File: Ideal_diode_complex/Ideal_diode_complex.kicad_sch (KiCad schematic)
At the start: 34 parts, among them CN1 24_243_1, CN2 24_243_1, CN3 24_243_2, CN4 24_243_2, Q1 SI7336ADP-T1-GE3-HXY, U1 TPS61041DBVR, U2 LTC4352CMS_TRPBF

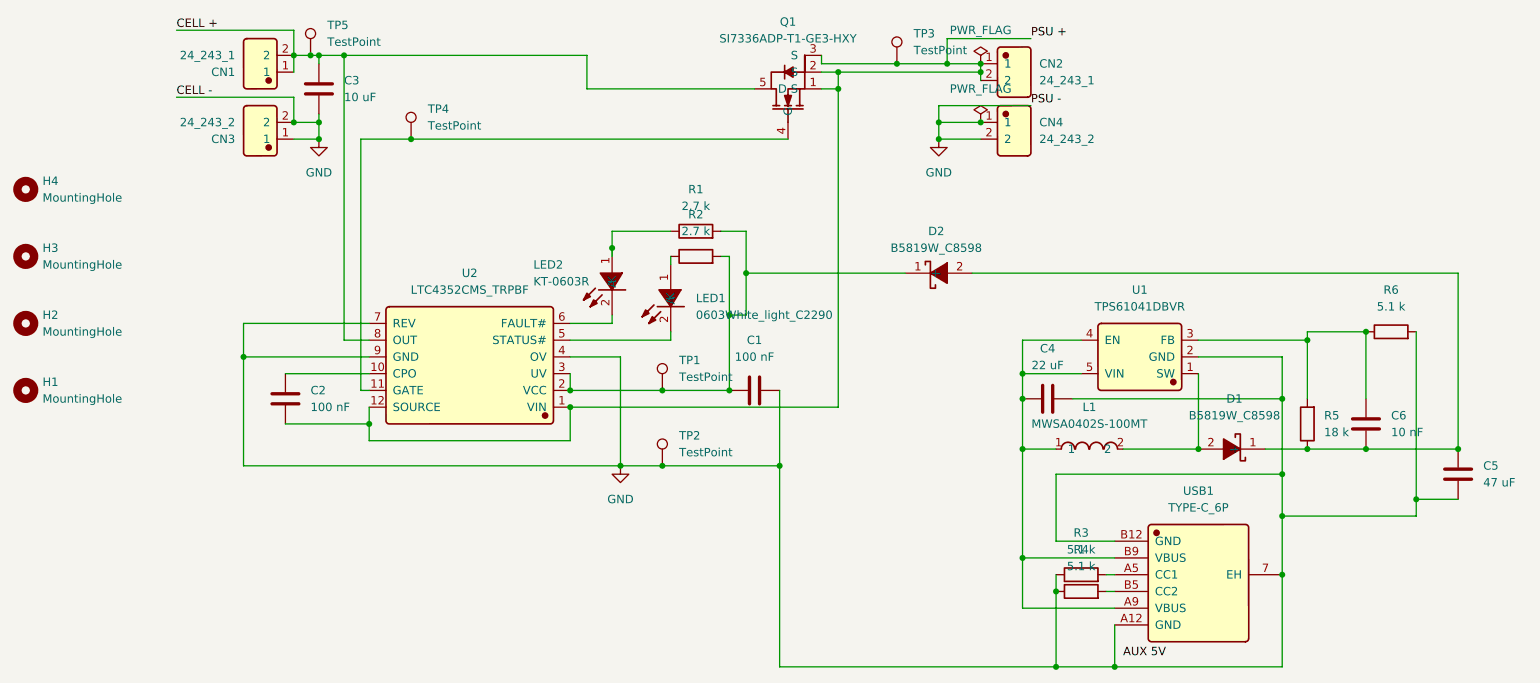
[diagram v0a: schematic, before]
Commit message: Final design
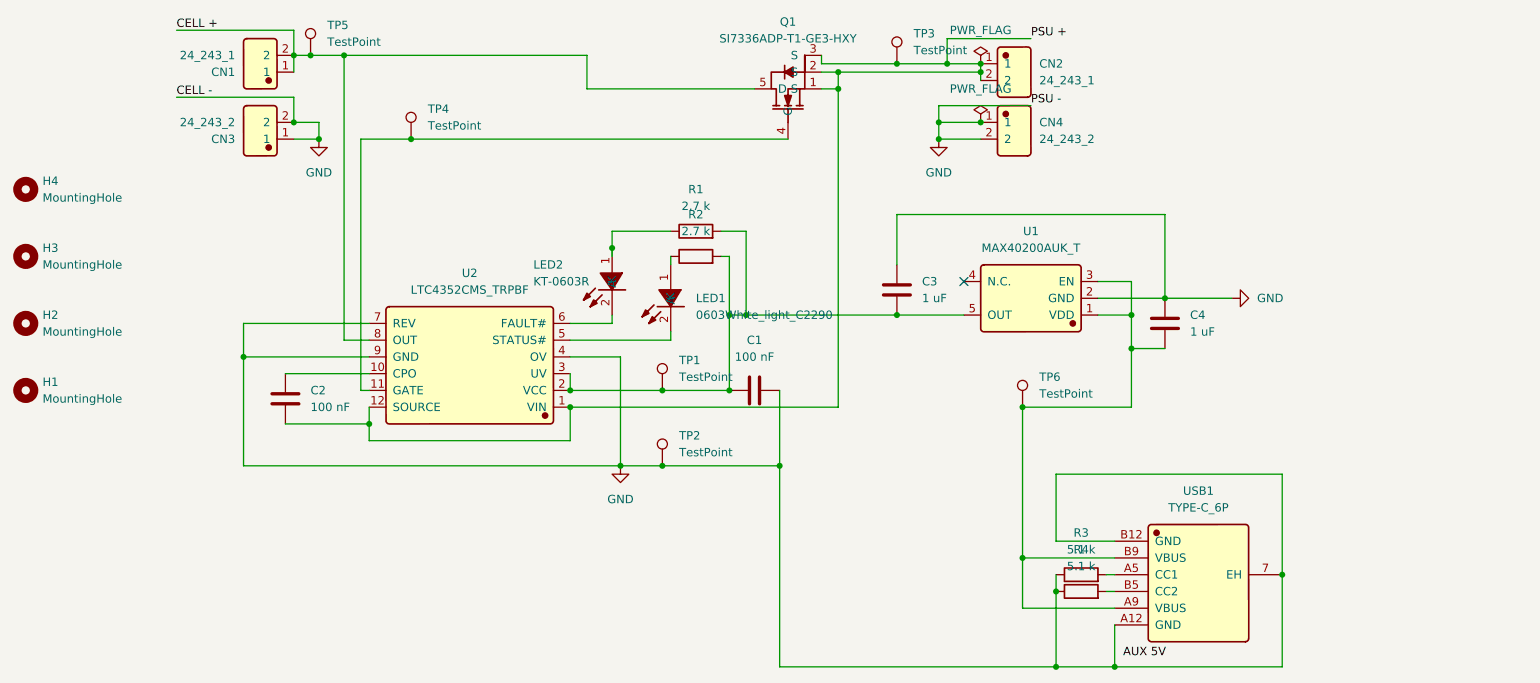
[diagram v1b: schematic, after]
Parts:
- removed C5: 47 uF, Capacitor_SMD:C_1206_3216Metric, symbol Device:C
- removed C6: 10 nF, Capacitor_SMD:C_0402_1005Metric, symbol Device:C
- removed D1, D2: B5819W_C8598, JLCImport:B5819W_C8598, symbol JLCImport:B5819W_C8598
- removed L1: MWSA0402S-100MT, JLCImport:MWSA0402S-100MT, symbol JLCImport:MWSA0402S-100MT
- removed R5: 18 k, Resistor_SMD:R_0603_1608Metric, symbol Device:R
- removed R6: 5.1 k, Resistor_SMD:R_0603_1608Metric, symbol Device:R
- removed U1: TPS61041DBVR, JLCImport:TPS61041DBVR, symbol JLCImport:TPS61041DBVR
- added TP6: TestPoint, TestPoint:TestPoint_Pad_D1.0mm, symbol Connector:TestPoint
- added U1: MAX40200AUK_T, JLCImport:MAX40200AUK_T, symbol JLCImport:MAX40200AUK_T
- C3: value 10 uF -> 1 uF; footprint Capacitor_SMD:C_1206_3216Metric -> Capacitor_SMD:C_0402_1005Metric
- C4: value 22 uF -> 1 uF; footprint Capacitor_SMD:C_1206_3216Metric -> Capacitor_SMD:C_0402_1005Metric
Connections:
- net CELL +: no longer C3.1
- net GND: now also C3.1, C4.1, U1.2 (GND); no longer C3.2, C4.2
- net at C1.1, R1.2, R2.2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: now also C3.2, U1.5 (OUT)
- net at USB1.A9 (VBUS), USB1.B9 (VBUS): now also C4.2, TP6.1, U1.1 (VDD), U1.3 (EN); no longer C4.1
- no-connect marks 0 -> 1
